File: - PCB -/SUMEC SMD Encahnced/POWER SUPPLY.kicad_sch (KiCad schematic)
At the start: 7 parts, among them U7 LM1084IS-5.0/NOPB, U8 LM1084IS-3.3/NOPB

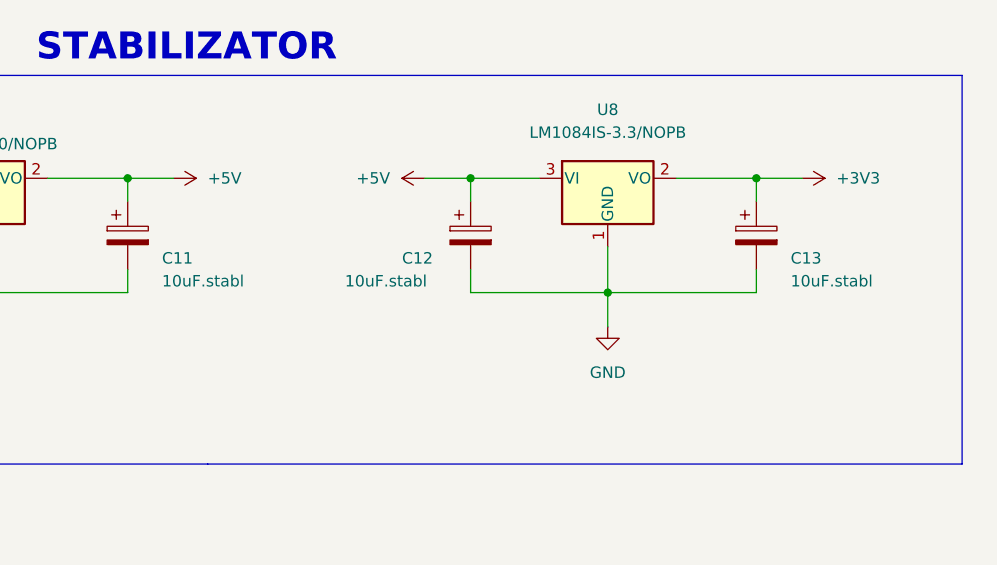
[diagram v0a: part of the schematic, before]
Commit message: QRE Array - WIP
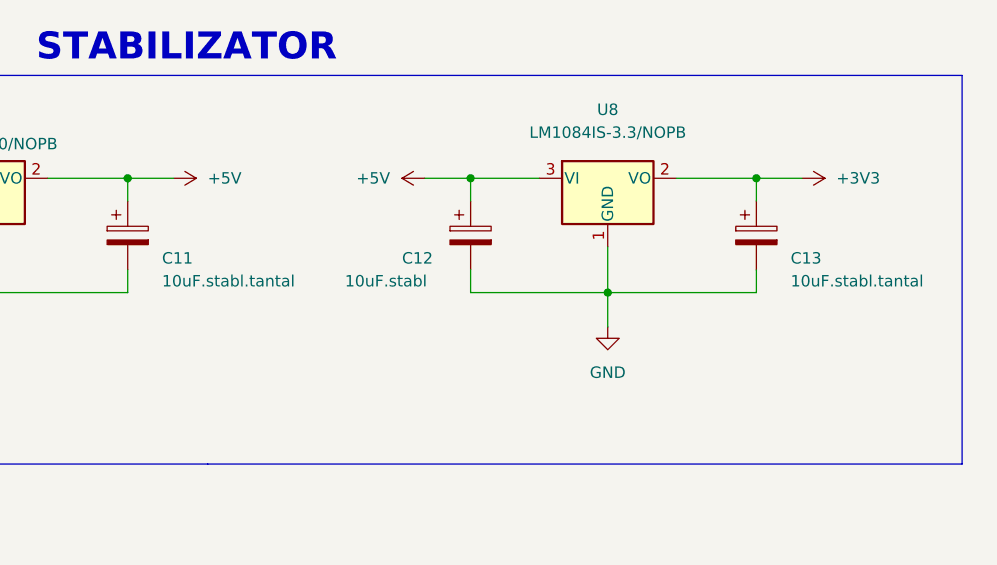
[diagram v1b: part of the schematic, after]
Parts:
- C11, C13: value 10uF.stabl -> 10uF.stabl.tantal
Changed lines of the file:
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@@
       (effects (font (size 1.27 1.27)) (justify left))
     )
-    (property "Value" "10uF.stabl" (at 139.7 55.88 0)
+    (property "Value" "10uF.stabl.tantal" (at 139.7 55.88 0)
       (effects (font (size 1.27 1.27)) (justify left))
     )
@@
       (effects (font (size 1.27 1.27)) (justify left))
     )
-    (property "Value" "10uF.stabl" (at 209.55 55.88 0)
+    (property "Value" "10uF.stabl.tantal" (at 209.55 55.88 0)
       (effects (font (size 1.27 1.27)) (justify left))
     )
